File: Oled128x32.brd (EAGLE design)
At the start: 31.2 x 11.9 mm, 18 parts, among them J1 1X04_SMD_STRAIGHT_COMBO

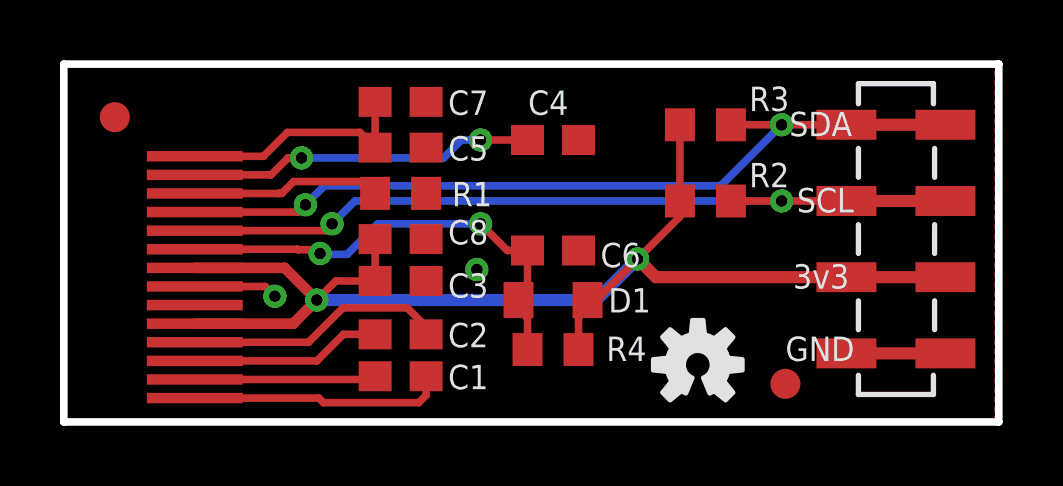
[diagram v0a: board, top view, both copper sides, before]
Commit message: Update Oled128x32.brd
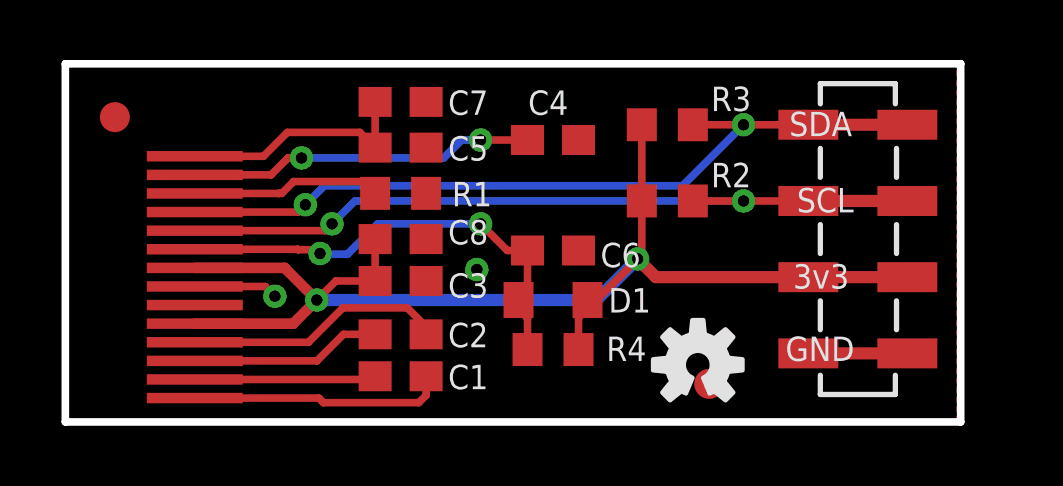
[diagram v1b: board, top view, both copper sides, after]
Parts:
- moved FD2 2.54 mm to (21.5, 1.27)
- moved J1 1.27 mm to (26.4, 2.29)
- moved R2 1.27 mm to (20.1, 7.37)
- moved R3 1.27 mm to (20.1, 9.91)
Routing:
- net +3V3: track 40.0 -> 38.2 mm
- net SCL: track 23.8 -> 22.6 mm
- net SDA: track 24.6 -> 23.3 mm
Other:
- board size 31.2 x 11.9 mm -> 29.8 x 11.9 mm
- board text added: "Oled128x32 rev. 1.1 psyte / Patrik Marcacci - 2019"
- board text removed: "Oled128x32 v1.0 psyte / Patrik Marcacci - 2018"
